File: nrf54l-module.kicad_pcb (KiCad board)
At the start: 4 copper layers, 16 x 25 mm, 137 parts, among them SW1 TS24CA, U1 NRF54L15-QFAA-R, U2 XL-0201SURC, U4 XL-0201SURC, U5 XL-0201SURC, U6 TLV62569DRLR, X1 XL7EL89CKI-111YLC-32M

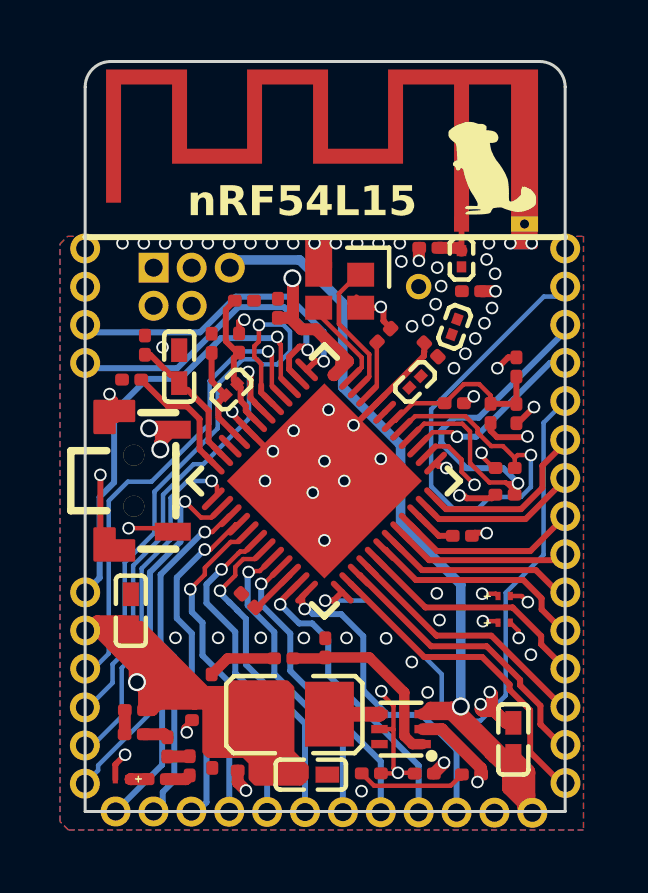
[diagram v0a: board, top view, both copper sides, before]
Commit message: chore: refactoring
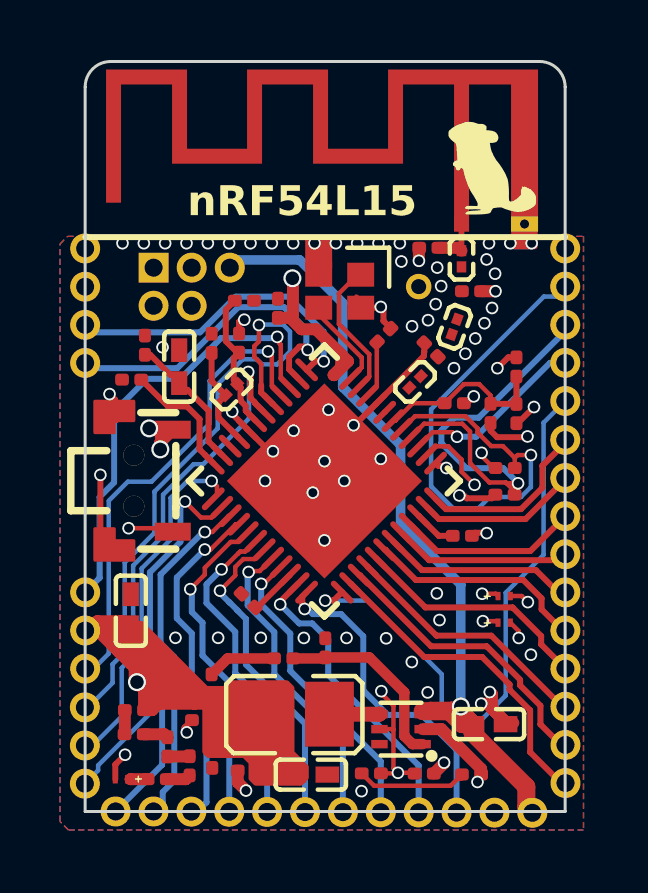
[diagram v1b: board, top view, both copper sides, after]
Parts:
- moved C17 0.96 mm to (39.3, 42.3), turned to 180 degrees
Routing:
- net VIN: track 38.6 -> 33.2 mm

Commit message: chore: refactoring
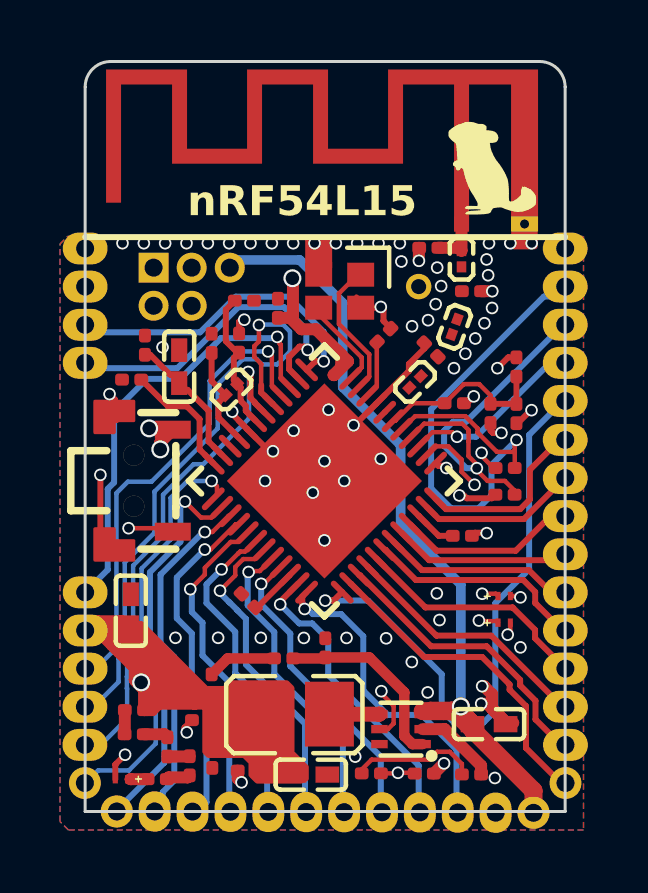
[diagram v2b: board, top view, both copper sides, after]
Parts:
- removed kibuzzard-68448C4F: G***, kibuzzard-68448C4F
- removed kibuzzard-68448C52: G***, kibuzzard-68448C52
- removed kibuzzard-68448C5C: G***, kibuzzard-68448C5C
- removed kibuzzard-68448C64: G***, kibuzzard-68448C64
- removed kibuzzard-68448C67: G***, kibuzzard-68448C67
- removed kibuzzard-684617F6: G***, kibuzzard-684617F6
- added kibuzzard-68463A68: G***, kibuzzard-68463A68, B.Cu at (27.7, 44.3)
- added kibuzzard-68463A73: G***, kibuzzard-68463A73, B.Cu at (27.8, 43.1)
- added kibuzzard-68463A78: G***, kibuzzard-68463A78, B.Cu at (27.8, 41.8)
- added kibuzzard-68463A7B: G***, kibuzzard-68463A7B, B.Cu at (27.8, 40.5)
- added kibuzzard-68463A81: G***, kibuzzard-68463A81, B.Cu at (27.8, 37.9)
- added kibuzzard-68463A85: G***, kibuzzard-68463A85, B.Cu at (27.2, 39.2)
- moved kibuzzard-68449000 0.54 mm to (28.5, 20.9)
- moved kibuzzard-68448B88 0.53 mm to (29.0, 23.1)
- moved kibuzzard-68461772 0.49 mm to (29.6, 22.0)
- moved kibuzzard-68449303 0.37 mm to (30.6, 43.1)
- moved kibuzzard-68449307 0.35 mm to (31.9, 43.1)
- moved kibuzzard-6844931D 0.34 mm to (36.9, 43.1)
- moved kibuzzard-6844930A 0.34 mm to (33.1, 43.1)
- moved kibuzzard-68449316 0.34 mm to (35.7, 43.1)
- moved kibuzzard-6844930F 0.33 mm to (34.4, 43.1)
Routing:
- net P0.03: track 15.2 -> 12.8 mm
- net nRESET: track 42.0 -> 40.7 mm
- net SW_EN: track 22.9 -> 24.2 mm
- net P1.00: track 13.3 -> 14.0 mm
- net Net-(R10-Pad1): track 3.61 -> 4.23 mm
